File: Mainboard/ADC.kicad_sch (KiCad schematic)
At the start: 23 parts, among them U10 TL072, U11 ADG419BR, U12 ADG419BR, U8 LTC2326CMS-16-PBF, U9 LT1469CS8-TRPBF

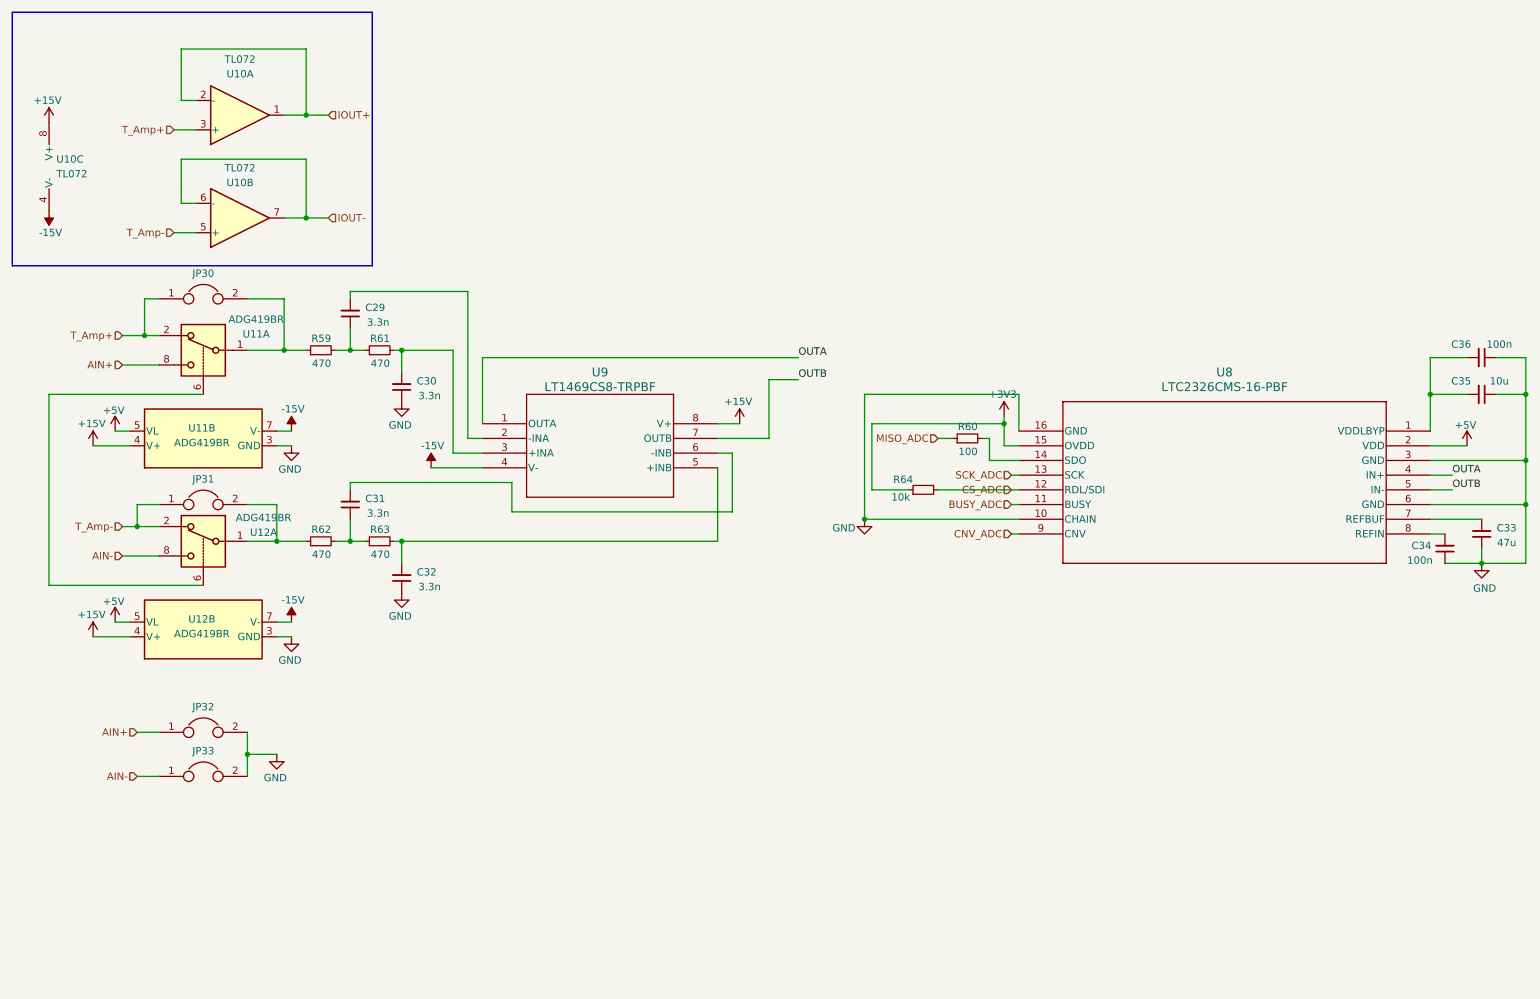
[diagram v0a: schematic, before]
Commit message: working mainboard push!
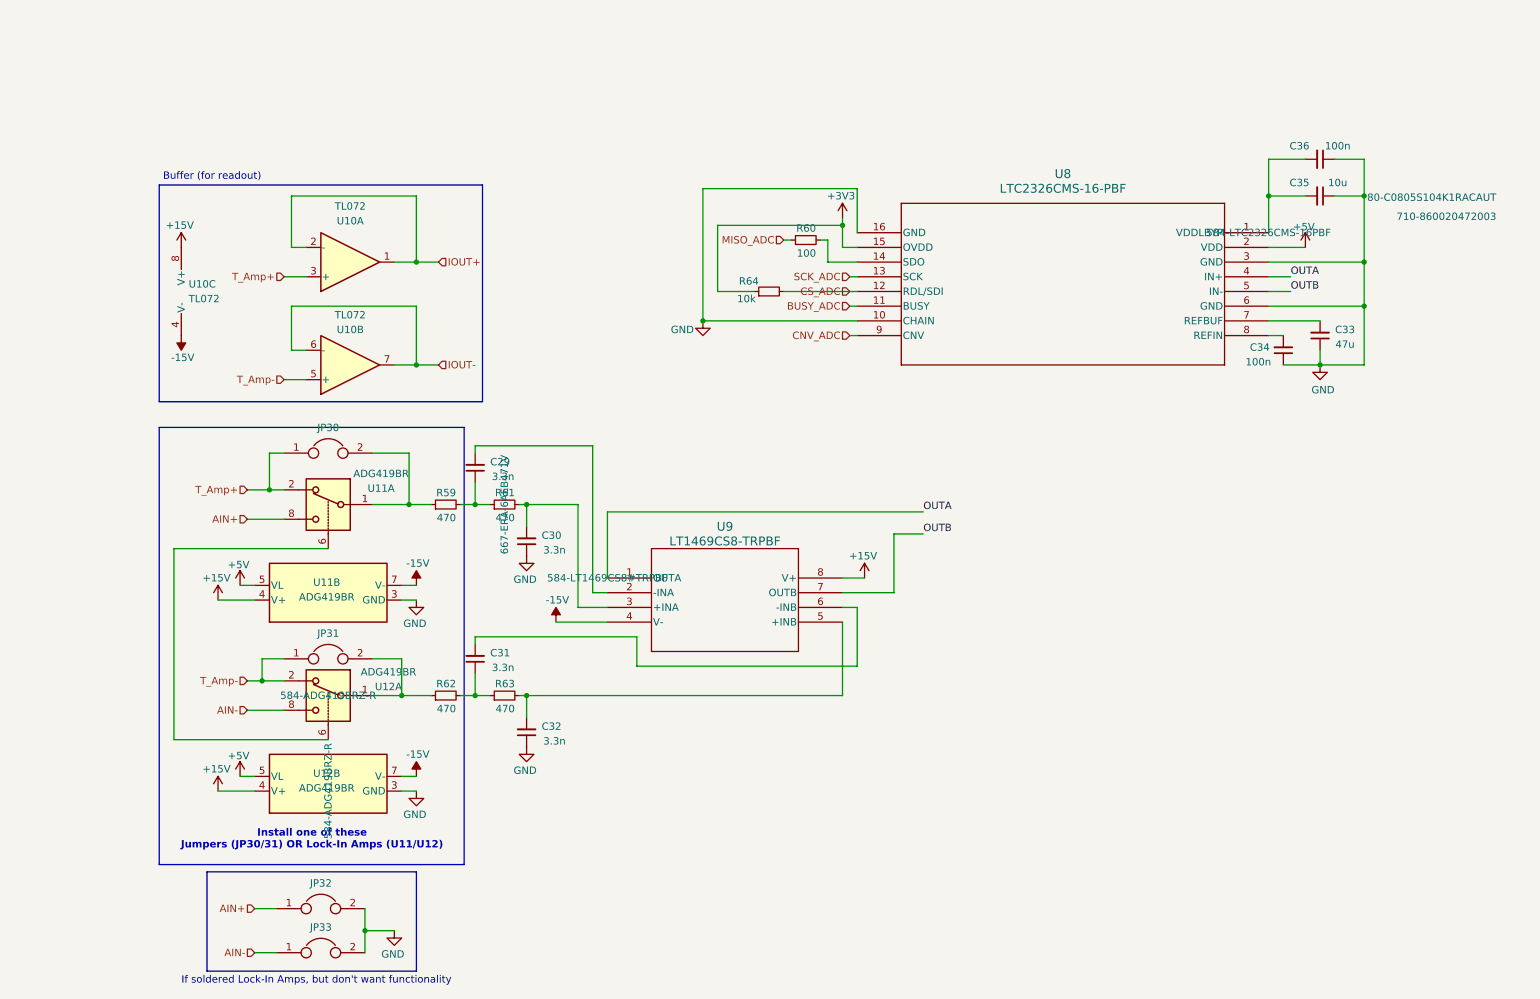
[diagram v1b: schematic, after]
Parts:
- C29, C30, C31, C32: footprint (none) -> Capacitor_SMD:C_0805_2012Metric; Mouser Part Number (none) -> 80-C0805C332KCR
- C33: footprint (none) -> Capacitor_SMD:C_0805_2012Metric; Mouser Part Number (none) -> 80-C0805C476M9P7800
- C34, C36: footprint (none) -> Capacitor_SMD:C_0805_2012Metric; Mouser Part Number (none) -> 80-C0805S104K1RACAUT
- C35: footprint (none) -> Capacitor_THT:CP_Radial_D5.0mm_P2.00mm; Mouser Part Number (none) -> 710-860020472003
- R59, R61, R62, R63: footprint (none) -> Resistor_SMD:R_0805_2012Metric; Mouser Part Number (none) -> 667-ERA-6AEB471V
- R60: footprint (none) -> Resistor_SMD:R_0805_2012Metric; Mouser Part Number (none) -> 708-RNCA0805BTE100R
- R64: footprint (none) -> Resistor_SMD:R_0805_2012Metric; Mouser Part Number (none) -> 755-ESR10EZPD1002
- U10: footprint (none) -> Package_SO:SOIC-8-1EP_3.9x4.9mm_P1.27mm_EP2.29x3mm_ThermalVias; Mouser Part Number (none) -> 511-TL072BIDT
- U11, U12: Mouser Part Number (none) -> 584-ADG419BRZ-R
- U8: Mouser Part Number (none) -> 584-LTC2326CMS-16PBF
- U9: Mouser Part Number (none) -> 584-LT1469CS8#TRPBF
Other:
- note added: "Buffer (for readout)"
- note added: "If soldered Lock-In Amps, but don't want functionality"
- note added: "Install one of these Jumpers (JP30/31) OR Lock-In Amps (U11/U12)"
- moved on the sheet: C29, C30, C31, C32, C33, C34, C35, C36, JP30, JP31, JP32, JP33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
